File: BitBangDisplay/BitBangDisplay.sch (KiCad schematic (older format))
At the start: 73 parts, among them J1 Conn_01x04, J11 Conn_01x01, J12 Conn_01x01, J13 KeyerJack, J14 KeyerJack, J15 KeyerJack, J16 SPEAKER, J2 Audio-Jack-3_2Switches, J20 Conn_01x01, J21 Conn_01x01, J3 Conn_01x01, J4 Conn_01x01, J5 Conn_01x01, J6 Conn_01x01, J7 Conn_01x01, J8 Conn_01x01, J9 Conn_01x01, SW2 SW_Push, SW3 SW_Push, SW4 SW_Push, SW5 SW_Push, U1 LCD1602ExtraPins, U2 LM358, U5 LCD1602ExtraPins

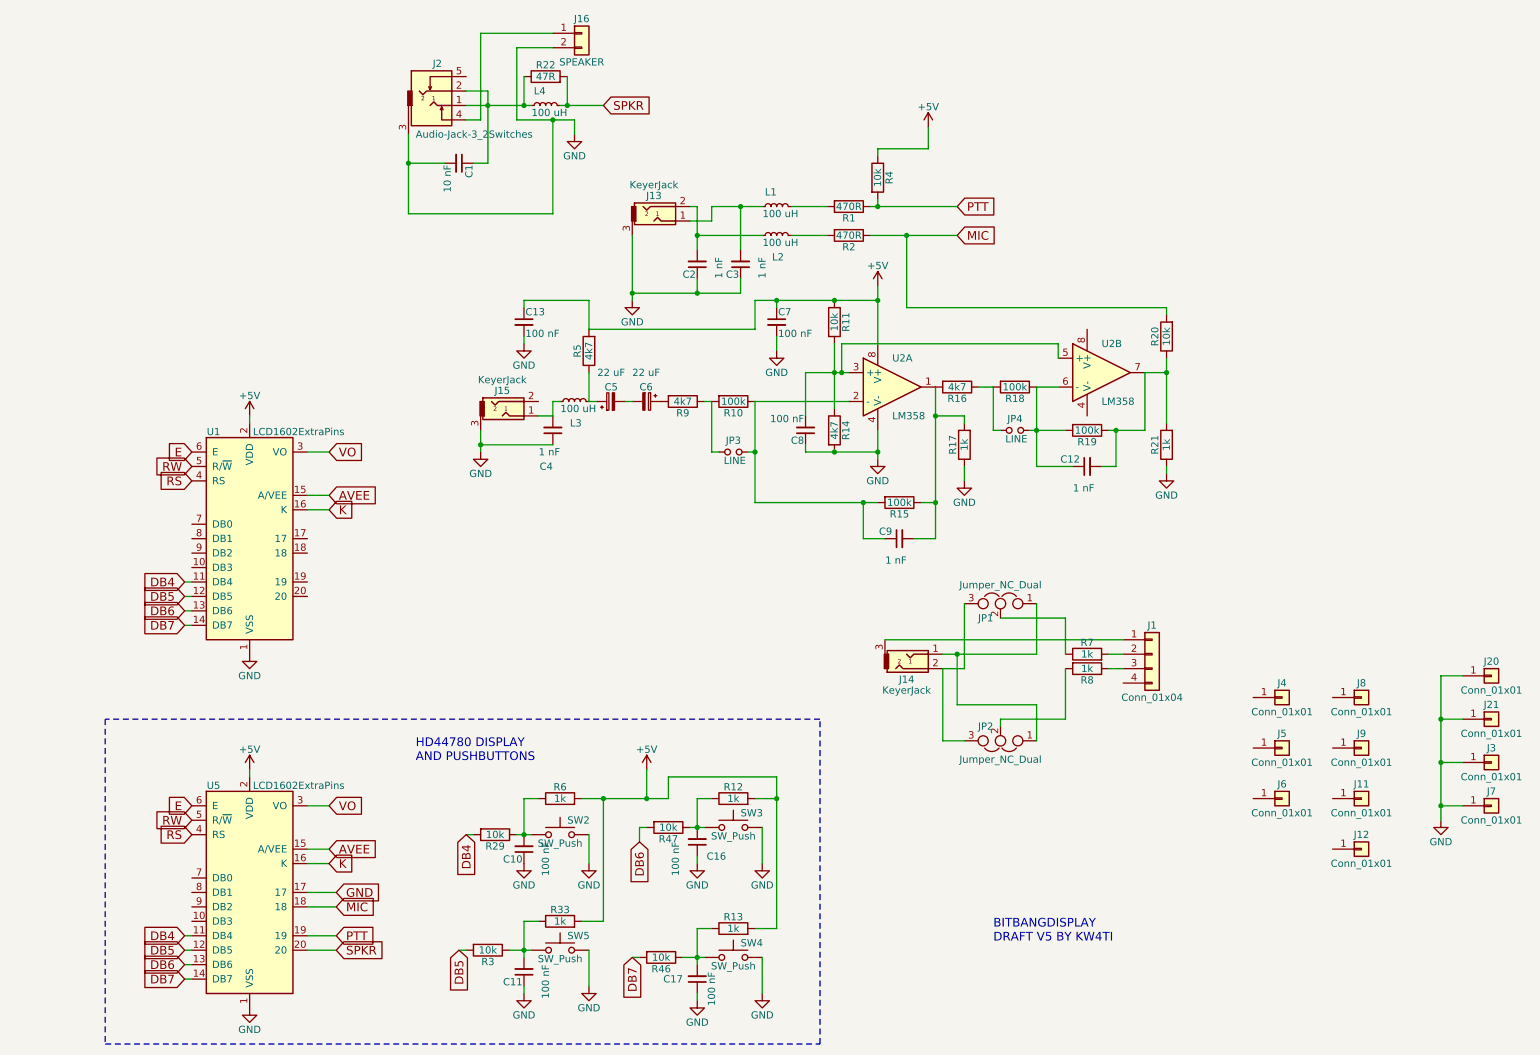
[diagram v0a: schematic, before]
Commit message: Added fifth button
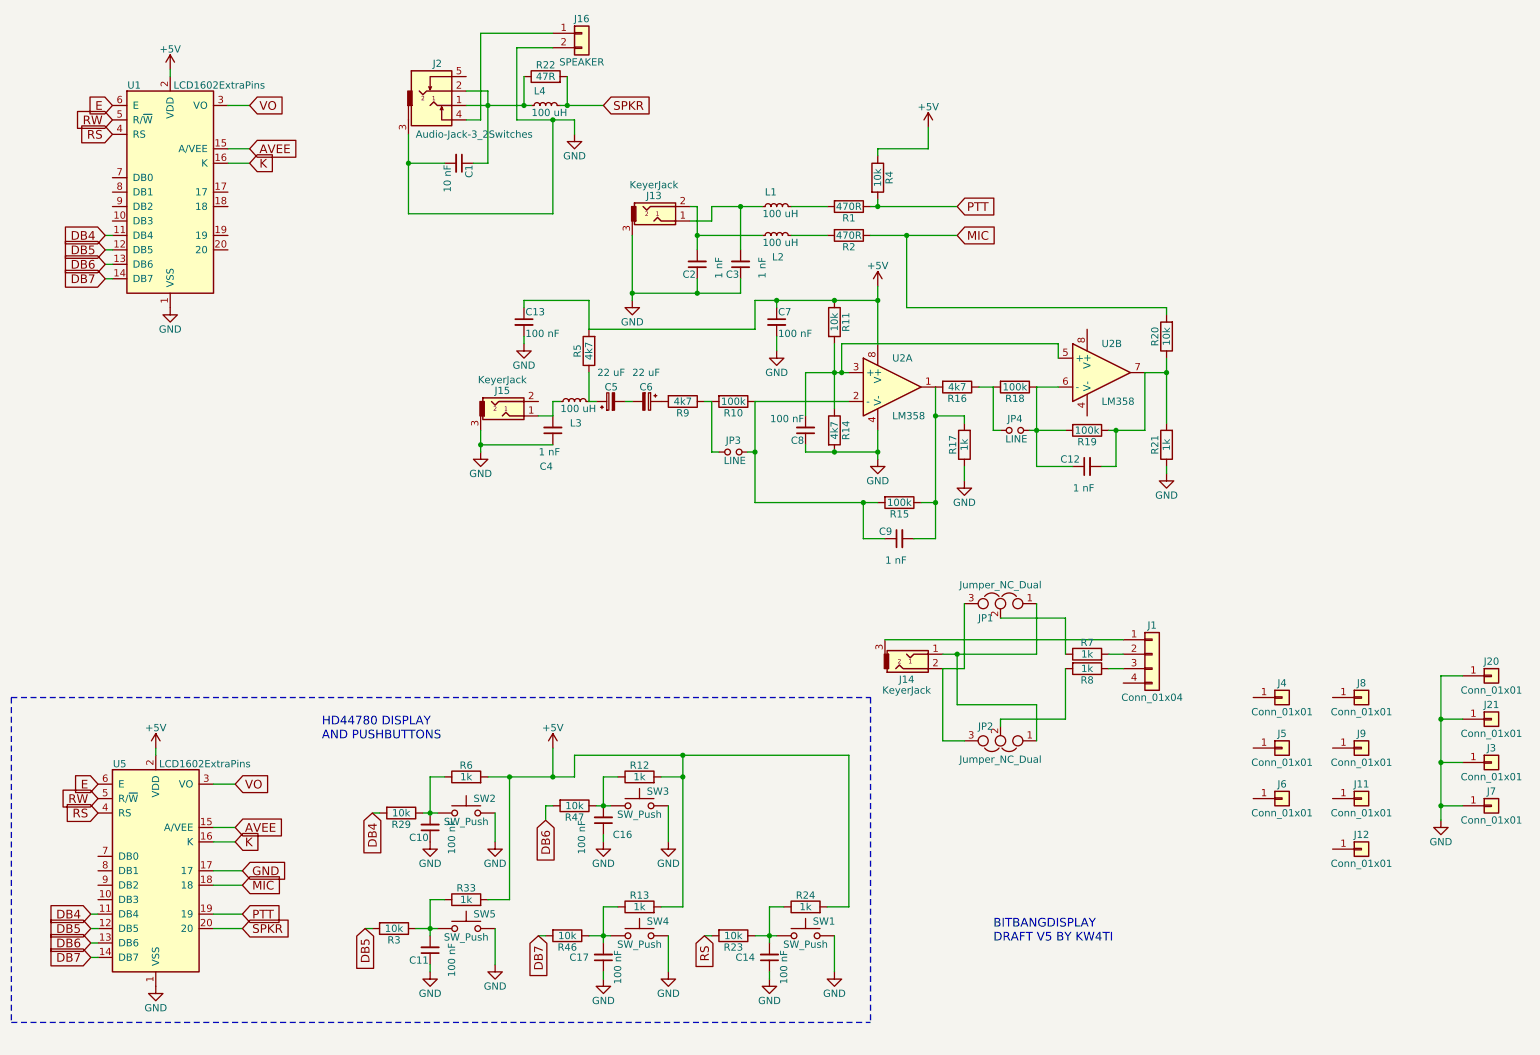
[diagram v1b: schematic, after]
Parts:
- added C14: 100 nF, Capacitors_THT:C_Disc_D5.0mm_W2.5mm_P2.50mm, symbol C_Small
- added R23: 10k, Resistors_THT:R_Axial_DIN0207_L6.3mm_D2.5mm_P7.62mm_Horizontal, symbol R
- added R24: 1k, Resistors_THT:R_Axial_DIN0207_L6.3mm_D2.5mm_P7.62mm_Horizontal, symbol R
- added SW1: SW_Push, Buttons_Switches_THT:SW_PUSH_6mm, symbol SW_Push
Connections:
- net +5V: now also R24.2
- net GND: now also C14.1, SW1.2
- net RS: now also R23.2
- new net: C14.2, R23.1, R24.1, SW1.1
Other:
- moved on the sheet: C10, C11, C16, C17, R12, R13, R29, R3, R33, R46, R47, R6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
